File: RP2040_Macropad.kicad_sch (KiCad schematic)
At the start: 54 parts, among them J1 External GPIOs, SW1 SW_Push, SW10 RotaryEncoder_Switch, SW11 SW_Push, SW12 SW_Push, SW2 SW_Push, SW3 SW_Push, SW4 SW_Push, SW5 SW_Push, SW6 SW_Push, SW7 SW_Push, SW8 SW_Push, SW9 SW_Push, U1 kb2040

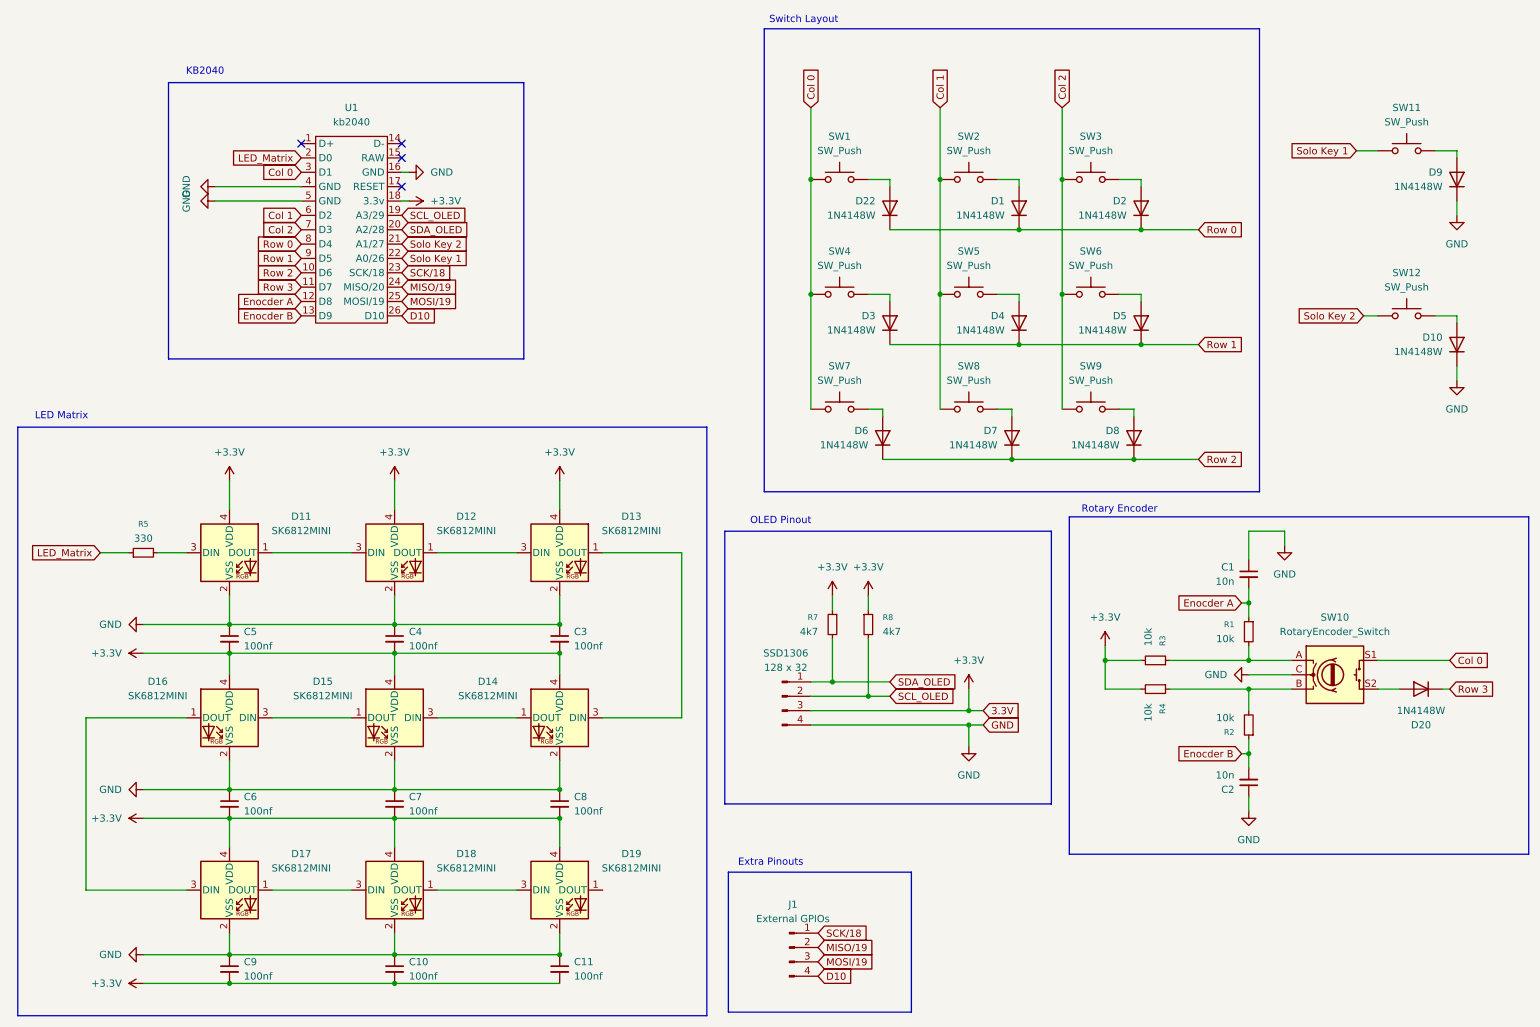
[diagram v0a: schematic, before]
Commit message: layout complete
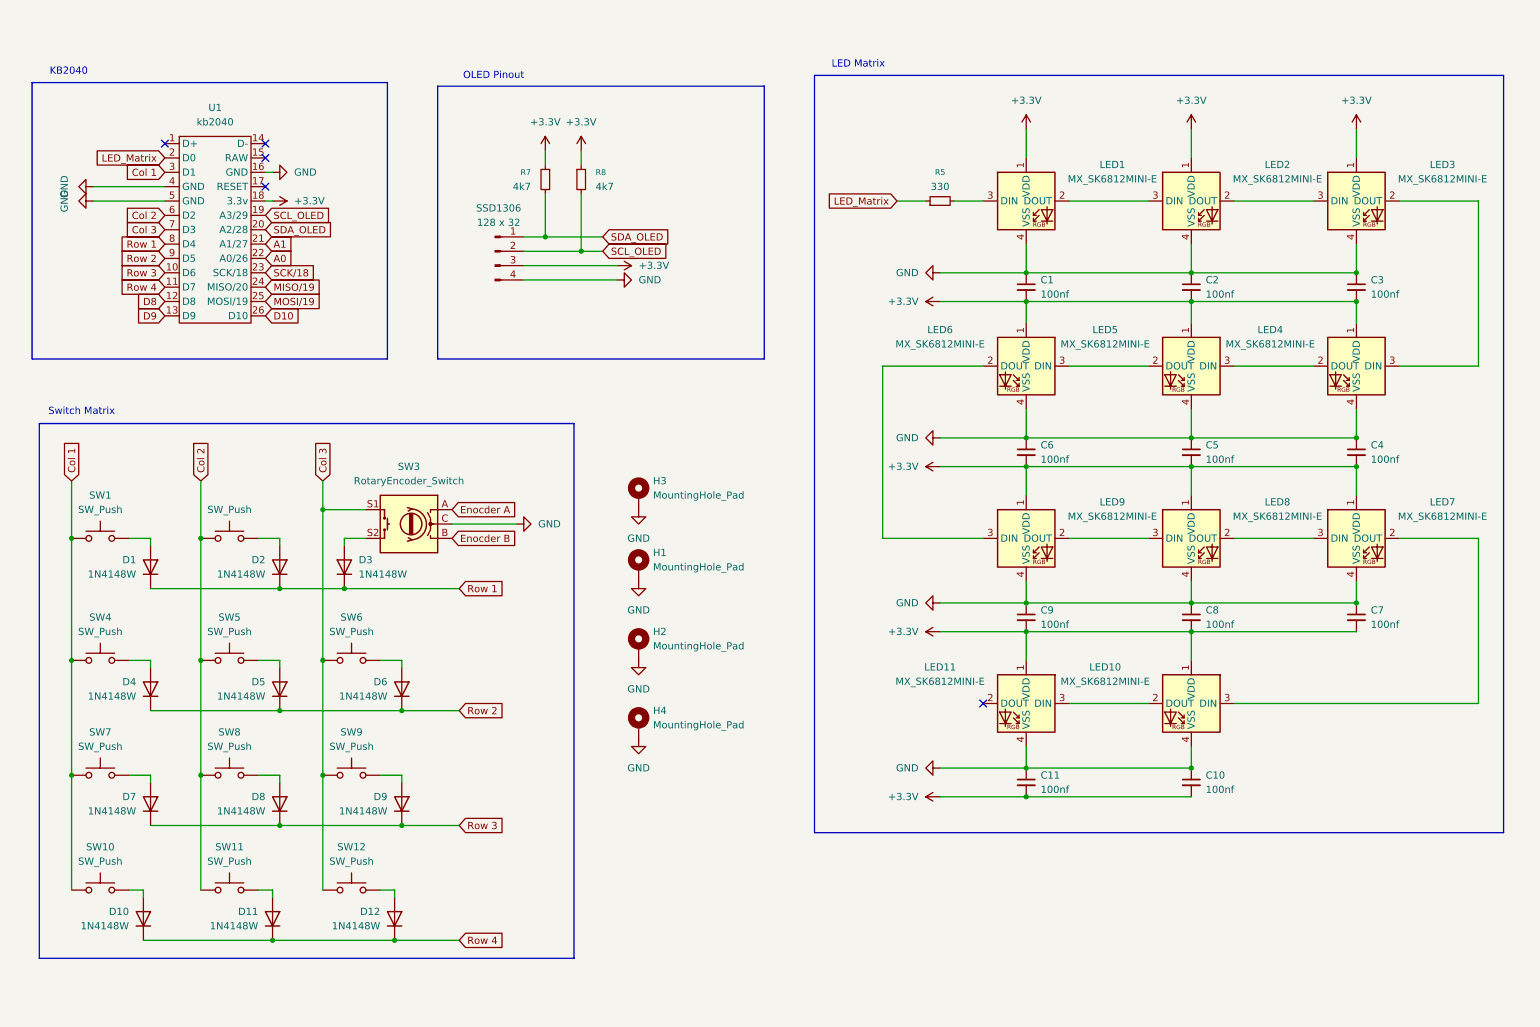
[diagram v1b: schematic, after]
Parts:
- removed C1, C2: 10n, Capacitor_SMD:C_0603_1608Metric, symbol Device:C_Small
- removed D11, D12, D13, D14, D15, D16, D17, D18, D19: SK6812MINI, LED_SMD:LED_SK6812MINI_PLCC4_3.5x3.5mm_P1.75mm, symbol LED:SK6812MINI
- removed D20, D22: 1N4148W, Diode_SMD:D_SOD-123, symbol Diode:1N4148W
- removed J1: External GPIOs, Connector_PinHeader_2.54mm:PinHeader_1x04_P2.54mm_Vertical, symbol Connector:Conn_01x04_Pin
- removed R1, R2, R3, R4: 10k, Resistor_SMD:R_0603_1608Metric, symbol Device:R_Small
- added C10, C11: 100nf, Capacitor_SMD:C_0603_1608Metric, symbol Device:C_Small
- added D3, D4: 1N4148W, Diode_SMD:D_SOD-123, symbol Diode:1N4148W
- added H1, H2, H3, H4: MountingHole_Pad, MountingHole:MountingHole_3.2mm_M3_DIN965_Pad, symbol Mechanical:MountingHole_Pad
- added LED1, LED10, LED11, LED2, LED3, LED4, LED5, LED6, LED7, LED8, LED9: MX_SK6812MINI-E, PCM_marbastlib-mx:LED_MX_6028R, symbol PCM_marbastlib-mx:MX_SK6812MINI-E
- renumbered C5 to C1, C4 to C2, C8 to C4, C7 to C5, C11 to C7, C10 to C8, D10 to D1, D6 to D10, D7 to D11, D8 to D12, D9 to D2, D1 to D5, D2 to D6, D3 to D7, D4 to D8, D5 to D9, SW12 to SW1, SW7 to SW10, SW8 to SW11, SW9 to SW12, SW11 to SW2, SW10 to SW3, SW1 to SW4, SW2 to SW5, SW3 to SW6, SW4 to SW7, SW5 to SW8, SW6 to SW9
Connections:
- net +3.3V: now also C10.2, C11.2, LED1.1 (VDD), LED10.1 (VDD), LED11.1 (VDD), LED2.1 (VDD), LED3.1 (VDD), LED4.1 (VDD), LED5.1 (VDD), LED6.1 (VDD), LED7.1 (VDD), LED8.1 (VDD), LED9.1 (VDD)
- net Col 1: now also SW1.1, SW10.1, SW4.1, SW7.1, U1.3 (D1); no longer SW11.1, SW5.1, SW8.1, U1.6 (D2)
- net Col 2: now also SW11.1, SW2.1, SW5.1, SW8.1, U1.6 (D2); no longer SW12.1, SW6.1, SW9.1, U1.7 (D3)
- net Enocder A: now also SW3.A; no longer U1.12 (D8)
- net Enocder B: now also SW3.B; no longer U1.13 (D9)
- net GND: now also C10.1, C11.1, H1.1, H2.1, H3.1, H4.1, LED1.4 (VSS), LED10.4 (VSS), LED11.4 (VSS), LED2.4 (VSS), LED3.4 (VSS), LED4.4 (VSS), LED5.4 (VSS), LED6.4 (VSS), LED7.4 (VSS), LED8.4 (VSS), LED9.4 (VSS); no longer D1.1 (K), D2.1 (K)
- net Row 1: now also D1.1 (K), D2.1 (K), U1.8 (D4), D3.1 (K); no longer D7.1 (K), D8.1 (K), D9.1 (K), U1.9 (D5)
- net Row 2: now also D5.1 (K), D6.1 (K), U1.9 (D5), D4.1 (K); no longer D10.1 (K), D11.1 (K), D12.1 (K), U1.10 (D6)
- net Row 3: now also D7.1 (K), D8.1 (K), D9.1 (K), U1.10 (D6); no longer U1.11 (D7)
- net at SW4.2: now also D4.2 (A)
- net at R5.2: now also LED1.3 (DIN)
- net at SW3.S2: now also D3.2 (A)
- removed net Col 0: SW10.1, SW3.S1, SW4.1, SW7.1, U1.3 (D1)
- removed net Row 0: D5.1 (K), D6.1 (K), U1.8 (D4)
- net Solo Key 1 renamed A0
- net A0: no longer SW2.1
- net Solo Key 2 renamed A1
- net A1: no longer SW1.1
- new net: LED1.2 (DOUT), LED2.3 (DIN)
- new net: LED4.2 (DOUT), LED5.3 (DIN)
- new net: LED3.2 (DOUT), LED4.3 (DIN)
- new net: LED10.3 (DIN), LED7.2 (DOUT)
- new net: LED7.3 (DIN), LED8.2 (DOUT)
- new net: LED2.2 (DOUT), LED3.3 (DIN)
- new net: LED10.2 (DOUT), LED11.3 (DIN)
- new net: LED8.3 (DIN), LED9.2 (DOUT)
- new net: LED6.2 (DOUT), LED9.3 (DIN)
- new net: LED5.2 (DOUT), LED6.3 (DIN)
- new net Col 3: SW12.1, SW3.S1, SW6.1, SW9.1, U1.7 (D3)
- new net D8: U1.12 (D8)
- new net D9: U1.13 (D9)
- new net Row 4: D10.1 (K), D11.1 (K), D12.1 (K), U1.11 (D7)
- no-connect marks 4 -> 5
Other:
- note added: "Switch Matrix"
- note removed: "Extra Pinouts"
- note removed: "Rotary Encoder"
- note removed: "Switch Layout"
- moved on the sheet: C1, C2, C3, C4, C5, C6, C7, C8, C9, D1, D10, D11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
